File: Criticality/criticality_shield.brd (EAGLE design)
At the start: 99 x 80 mm, 28 parts

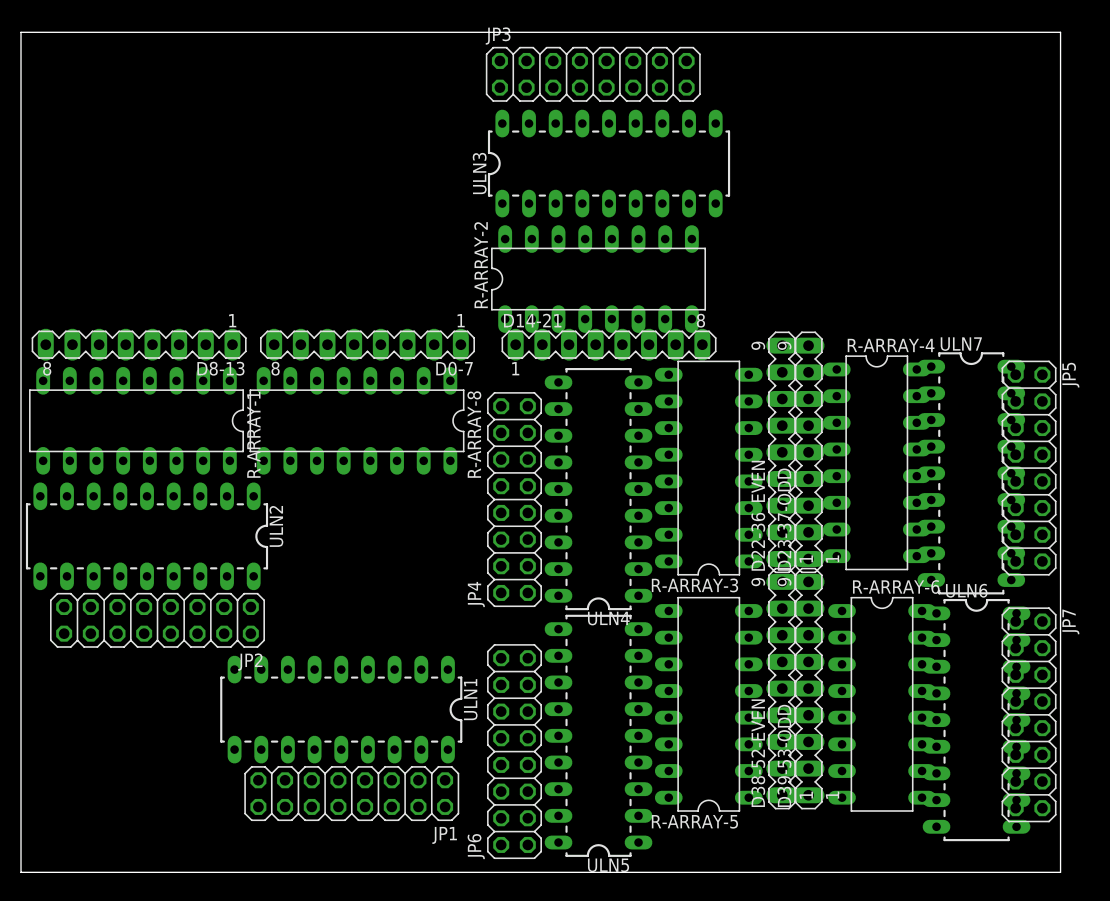
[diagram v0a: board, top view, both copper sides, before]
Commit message: completely new version (SMD)
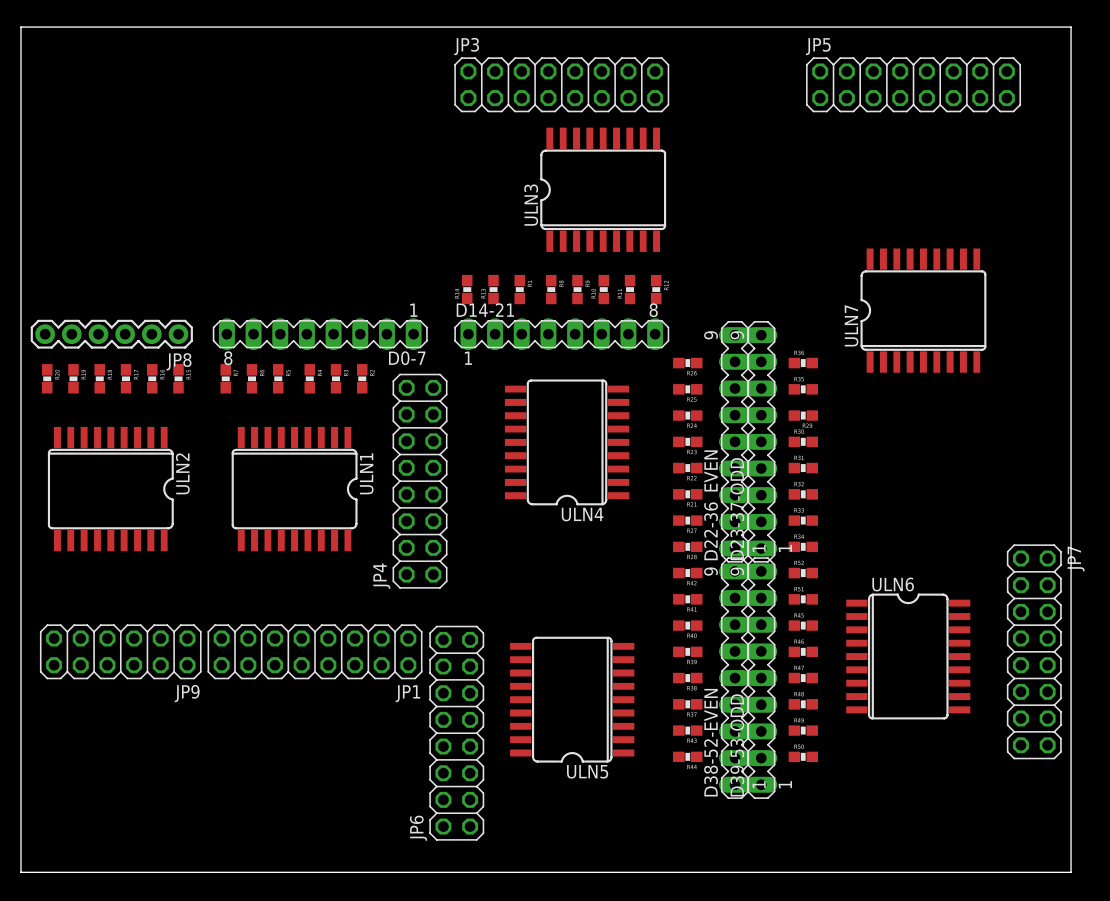
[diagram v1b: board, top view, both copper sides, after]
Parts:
- removed D8-13: (no value), con-lstb:MA08-1
- removed JP2: (no value), pinhead:2X08
- removed R-ARRAY-1, R-ARRAY-2, R-ARRAY-3, R-ARRAY-4, R-ARRAY-5, R-ARRAY-6, R-ARRAY-8: (no value), ic-package:DIL16
- added JP8: (no value), SparkFun-Connectors:1X06
- added JP9: (no value), pinhead:2X06
- added R1, R10, R11, R12, R13, R14, R15, R16, R17, R18, R19, R2, R20, R21, R22, R23, R24, R25, R26, R27, R28, R29, R3, R30, R31, R32, R33, R34, R35, R36, R37, R38, R39, R4, R40, R41, R42, R43, R44, R45, R46, R47, R48, R49, R5, R50, R51, R52, R6, R7, R8, R9: (no value), SparkFun-Resistors:0603-RES
- ULN1, ULN2, ULN3, ULN4, ULN5, ULN6, ULN7: value ULN2803 -> (none); device SparkFun-PowerIC:DIL18 -> SparkFun-PowerIC:SO18L
- moved JP5 38.1 mm to (85.0, 75.0), turned to 0 degrees
- moved ULN1 21.0 mm to (30.5, 36.5)
- moved ULN7 17.9 mm to (81.5, 53.5), turned to 0 degrees
- moved JP1 13.9 mm to (28.0, 21.0)
- moved ULN6 12.3 mm to (84.5, 25.0)
- moved JP4 9.17 mm to (38.0, 37.2)
- moved JP7 6.02 mm to (96.5, 21.0)
- moved JP6 5.77 mm to (41.5, 13.2)
- moved ULN3 5.59 mm to (51.0, 65.0)
- moved D0-7 4.61 mm to (28.5, 51.2)
- moved D14-21 4.61 mm to (51.5, 51.2)
- moved D22-36_EVEN 4.61 mm to (68.0, 41.0)
- moved D23-37-ODD 4.61 mm to (70.5, 41.0)
- moved D38-52-EVEN 4.61 mm to (68.0, 18.5)
- moved D39-53-ODD 4.61 mm to (70.5, 18.5)
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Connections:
- removed net N$11 (its old number): R-ARRAY-8.14, ULN1.3
- removed net N$12 (its old number): R-ARRAY-8.13, ULN1.4
- removed net N$122 (its old number): JP2.3, ULN2.17
- removed net N$123 (its old number): JP2.5, ULN2.16
- removed net N$124 (its old number): JP2.7, ULN2.15
- removed net N$125 (its old number): JP2.9, ULN2.14
- removed net N$126 (its old number): JP2.11, ULN2.13
- removed net N$17: R-ARRAY-1.16, ULN2.1
- removed net N$33 (its old number): R-ARRAY-2.14, ULN3.3
- removed net N$34 (its old number): R-ARRAY-2.13, ULN3.4
- removed net N$66 (its old number): R-ARRAY-8.12, ULN1.5
- removed net N$67 (its old number): R-ARRAY-8.11, ULN1.6
- new net N$107: R5.2, ULN1.6
- new net N$108: R4.2, ULN1.5
- new net N$109: R3.2, ULN1.4
- new net N$110: R2.2, ULN1.3
- new net N$133: R20.2, ULN2.8
- new net N$134: R19.2, ULN2.7
- new net N$159: R18.2, ULN2.6
- new net N$160: R17.2, ULN2.5
- new net N$161: R16.2, ULN2.4
- new net N$162: R15.2, ULN2.3
- net +5V: now also JP9.10, JP9.12, JP9.2, JP9.4, JP9.6, JP9.8; no longer JP2.10, JP2.12, JP2.14, JP2.16, JP2.2, JP2.4, JP2.6, JP2.8
- net GND: no longer D8-13.7
- net N$1: now also R2.1; no longer R-ARRAY-8.1
- net N$10: now also R14.2, ULN3.1; no longer R-ARRAY-8.15, ULN1.2
- net N$100: now also D39-53-ODD.6, R46.1; no longer R-ARRAY-6.13, ULN6.4
- net N$101: now also D39-53-ODD.5, R47.1; no longer R-ARRAY-6.12, ULN6.5
- net N$102: now also D39-53-ODD.4, R48.1; no longer R-ARRAY-6.11, ULN6.6
- net N$103: now also D39-53-ODD.3, R49.1; no longer R-ARRAY-6.10, ULN6.7
- net N$104: now also D39-53-ODD.2, R50.1; no longer R-ARRAY-6.9, ULN6.8
- net N$105: now also R7.2, ULN1.8; no longer JP1.1, ULN1.18
- net N$106: now also R6.2, ULN1.7; no longer JP1.3, ULN1.17
- net N$111: now also R8.2, ULN3.4; no longer JP1.13
- net N$112: now also R1.2, ULN3.3; no longer JP1.15
- net N$121: now also JP9.11, ULN2.11; no longer JP2.1, ULN2.18
- net N$13: now also JP8.TXO, R17.1; no longer D8-13.3, R-ARRAY-1.3
- net N$14: now also JP8.VCC, R18.1; no longer D8-13.4, R-ARRAY-1.4
- net N$15: now also JP8.CTS, R19.1; no longer D8-13.5, R-ARRAY-1.5
- net N$16: now also JP8.GND, R20.1; no longer D8-13.6, R-ARRAY-1.6
- net N$18: now also JP9.1, ULN2.16; no longer R-ARRAY-1.15, ULN2.2
- net N$19: now also JP9.3, ULN2.15; no longer R-ARRAY-1.14, ULN2.3
- net N$2: now also R3.1; no longer R-ARRAY-8.2
- net N$20: now also R14.1; no longer R-ARRAY-2.1
- net N$21: now also R13.1; no longer R-ARRAY-2.2
- net N$22: now also R1.1; no longer R-ARRAY-2.3
- net N$23: now also R8.1; no longer R-ARRAY-2.4
- net N$24: now also JP9.5, ULN2.14; no longer R-ARRAY-1.13, ULN2.4
- net N$25: now also JP9.7, ULN2.13; no longer R-ARRAY-1.12, ULN2.5
- net N$26: now also JP9.9, ULN2.12; no longer R-ARRAY-1.11, ULN2.6
- net N$27: now also R9.1; no longer R-ARRAY-2.5
- net N$28: now also R10.1; no longer R-ARRAY-2.6
- net N$29: now also JP1.13, ULN1.12; no longer D14-21.7, R-ARRAY-2.7
- net N$3: now also R4.1; no longer R-ARRAY-8.3
- net N$30: now also JP1.15, ULN1.11; no longer D14-21.8, R-ARRAY-2.8
- net N$31: now also D14-21.7, R11.1; no longer R-ARRAY-2.16, ULN3.1
- net N$32: now also D14-21.8, R12.1; no longer R-ARRAY-2.15, ULN3.2
- net N$35: now also R26.2, ULN4.8; no longer D22-36_EVEN.1, R-ARRAY-3.1
- net N$36: now also R25.2, ULN4.7; no longer D22-36_EVEN.2, R-ARRAY-3.2
- net N$37: now also R12.2, ULN3.8; no longer R-ARRAY-2.12, ULN3.5
- net N$38: now also R11.2, ULN3.7; no longer R-ARRAY-2.11, ULN3.6
- net N$39: now also R24.2, ULN4.6; no longer D22-36_EVEN.3, R-ARRAY-3.3
- net N$4: now also R5.1; no longer R-ARRAY-8.4
- net N$40: now also R23.2, ULN4.5; no longer D22-36_EVEN.4, R-ARRAY-3.4
- net N$41: now also R22.2, ULN4.4; no longer D22-36_EVEN.5, R-ARRAY-3.5
- net N$42: now also R21.2, ULN4.3; no longer D22-36_EVEN.6, R-ARRAY-3.6
- net N$43: now also R10.2, ULN3.6; no longer R-ARRAY-2.10, ULN3.7
- net N$44: now also R9.2, ULN3.5; no longer R-ARRAY-2.9, ULN3.8
- net N$45: now also R27.2, ULN4.2; no longer D22-36_EVEN.7, R-ARRAY-3.7
- net N$46: now also R28.2, ULN4.1; no longer D22-36_EVEN.8, R-ARRAY-3.8
- net N$47: now also D22-36_EVEN.1, R28.1; no longer R-ARRAY-3.16, ULN4.1
- net N$48: now also D22-36_EVEN.2, R27.1; no longer R-ARRAY-3.15, ULN4.2
- net N$49: now also D22-36_EVEN.3, R21.1; no longer R-ARRAY-3.14, ULN4.3
- net N$5: now also JP8.DTR, R15.1; no longer D8-13.1, R-ARRAY-1.1
- net N$50: now also D22-36_EVEN.4, R22.1; no longer R-ARRAY-3.13, ULN4.4
- net N$51: now also R34.2, ULN7.8; no longer D23-37-ODD.8, R-ARRAY-4.1
- net N$52: now also R33.2, ULN7.7; no longer D23-37-ODD.7, R-ARRAY-4.2
- net N$53: now also D22-36_EVEN.5, R23.1; no longer R-ARRAY-3.12, ULN4.5
- net N$54: now also D22-36_EVEN.6, R24.1; no longer R-ARRAY-3.11, ULN4.6
- net N$55: now also D22-36_EVEN.7, R25.1; no longer R-ARRAY-3.10, ULN4.7
- net N$56: now also D22-36_EVEN.8, R26.1; no longer R-ARRAY-3.9, ULN4.8
- net N$57: now also R32.2, ULN7.6; no longer D23-37-ODD.6, R-ARRAY-4.3
- net N$58: now also R31.2, ULN7.5; no longer D23-37-ODD.5, R-ARRAY-4.4
- net N$59: now also R30.2, ULN7.4; no longer D23-37-ODD.4, R-ARRAY-4.5
- net N$6: now also JP8.RXI, R16.1; no longer D8-13.2, R-ARRAY-1.2
- net N$60: now also R29.2, ULN7.3; no longer D23-37-ODD.3, R-ARRAY-4.6
- net N$61: now also R35.2, ULN7.2; no longer D23-37-ODD.2, R-ARRAY-4.7
- net N$62: now also R36.2, ULN7.1; no longer D23-37-ODD.1, R-ARRAY-4.8
- net N$63: now also D23-37-ODD.8, R36.1; no longer R-ARRAY-4.16, ULN7.1
- net N$64: now also D23-37-ODD.7, R35.1; no longer R-ARRAY-4.15, ULN7.2
- net N$65: now also D23-37-ODD.6, R29.1; no longer R-ARRAY-4.14, ULN7.3
- net N$68: now also D23-37-ODD.5, R30.1; no longer R-ARRAY-4.13, ULN7.4
- net N$69: now also D23-37-ODD.4, R31.1; no longer R-ARRAY-4.12, ULN7.5
- net N$7: now also R6.1; no longer R-ARRAY-8.5
- net N$70: now also R42.2, ULN5.8; no longer D38-52-EVEN.2, R-ARRAY-5.1
- net N$71: now also R41.2, ULN5.7; no longer D38-52-EVEN.3, R-ARRAY-5.2
- net N$72: now also R40.2, ULN5.6; no longer D38-52-EVEN.4, R-ARRAY-5.3
- net N$73: now also R39.2, ULN5.5; no longer D38-52-EVEN.5, R-ARRAY-5.4
- net N$74: now also R38.2, ULN5.4; no longer D38-52-EVEN.6, R-ARRAY-5.5
- net N$75: now also R37.2, ULN5.3; no longer D38-52-EVEN.7, R-ARRAY-5.6
- net N$76: now also R43.2, ULN5.2; no longer D38-52-EVEN.8, R-ARRAY-5.7
- net N$77: now also R44.2, ULN5.1; no longer D38-52-EVEN.9, R-ARRAY-5.8
- net N$78: now also D38-52-EVEN.2, R44.1; no longer R-ARRAY-5.16, ULN5.1
- net N$79: now also D38-52-EVEN.3, R43.1; no longer R-ARRAY-5.15, ULN5.2
- net N$8: now also R7.1; no longer R-ARRAY-8.6
- net N$80: now also D38-52-EVEN.4, R37.1; no longer R-ARRAY-5.14, ULN5.3
- net N$81: now also D38-52-EVEN.5, R38.1; no longer R-ARRAY-5.13, ULN5.4
- net N$82: now also D23-37-ODD.3, R32.1; no longer R-ARRAY-4.11, ULN7.6
- net N$83: now also D23-37-ODD.2, R33.1; no longer R-ARRAY-4.10, ULN7.7
- net N$84: now also D23-37-ODD.1, R34.1; no longer R-ARRAY-4.9, ULN7.8
- net N$85: now also D38-52-EVEN.6, R39.1; no longer R-ARRAY-5.12, ULN5.5
- net N$86: now also D38-52-EVEN.7, R40.1; no longer R-ARRAY-5.11, ULN5.6
- net N$87: now also D38-52-EVEN.8, R41.1; no longer R-ARRAY-5.10, ULN5.7
- net N$88: now also D38-52-EVEN.9, R42.1; no longer R-ARRAY-5.9, ULN5.8
- net N$89: now also R50.2, ULN6.8; no longer D39-53-ODD.9, R-ARRAY-6.1
- net N$9: now also R13.2, ULN3.2; no longer R-ARRAY-8.16, ULN1.1
- net N$90: now also R49.2, ULN6.7; no longer D39-53-ODD.8, R-ARRAY-6.2
- net N$91: now also R48.2, ULN6.6; no longer D39-53-ODD.7, R-ARRAY-6.3
- net N$92: now also R47.2, ULN6.5; no longer D39-53-ODD.6, R-ARRAY-6.4
- net N$93: now also R46.2, ULN6.4; no longer D39-53-ODD.5, R-ARRAY-6.5
- net N$94: now also R45.2, ULN6.3; no longer D39-53-ODD.4, R-ARRAY-6.6
- net N$95: now also R51.2, ULN6.2; no longer D39-53-ODD.3, R-ARRAY-6.7
- net N$96: now also R52.2, ULN6.1; no longer D39-53-ODD.2, R-ARRAY-6.8
- net N$97: now also D39-53-ODD.9, R52.1; no longer R-ARRAY-6.16, ULN6.1
- net N$98: now also D39-53-ODD.8, R51.1; no longer R-ARRAY-6.15, ULN6.2
- net N$99: now also D39-53-ODD.7, R45.1; no longer R-ARRAY-6.14, ULN6.3
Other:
- board size 99 x 80 mm -> 100 x 80.5 mm
